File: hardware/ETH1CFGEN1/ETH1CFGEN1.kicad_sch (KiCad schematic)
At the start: 0 parts

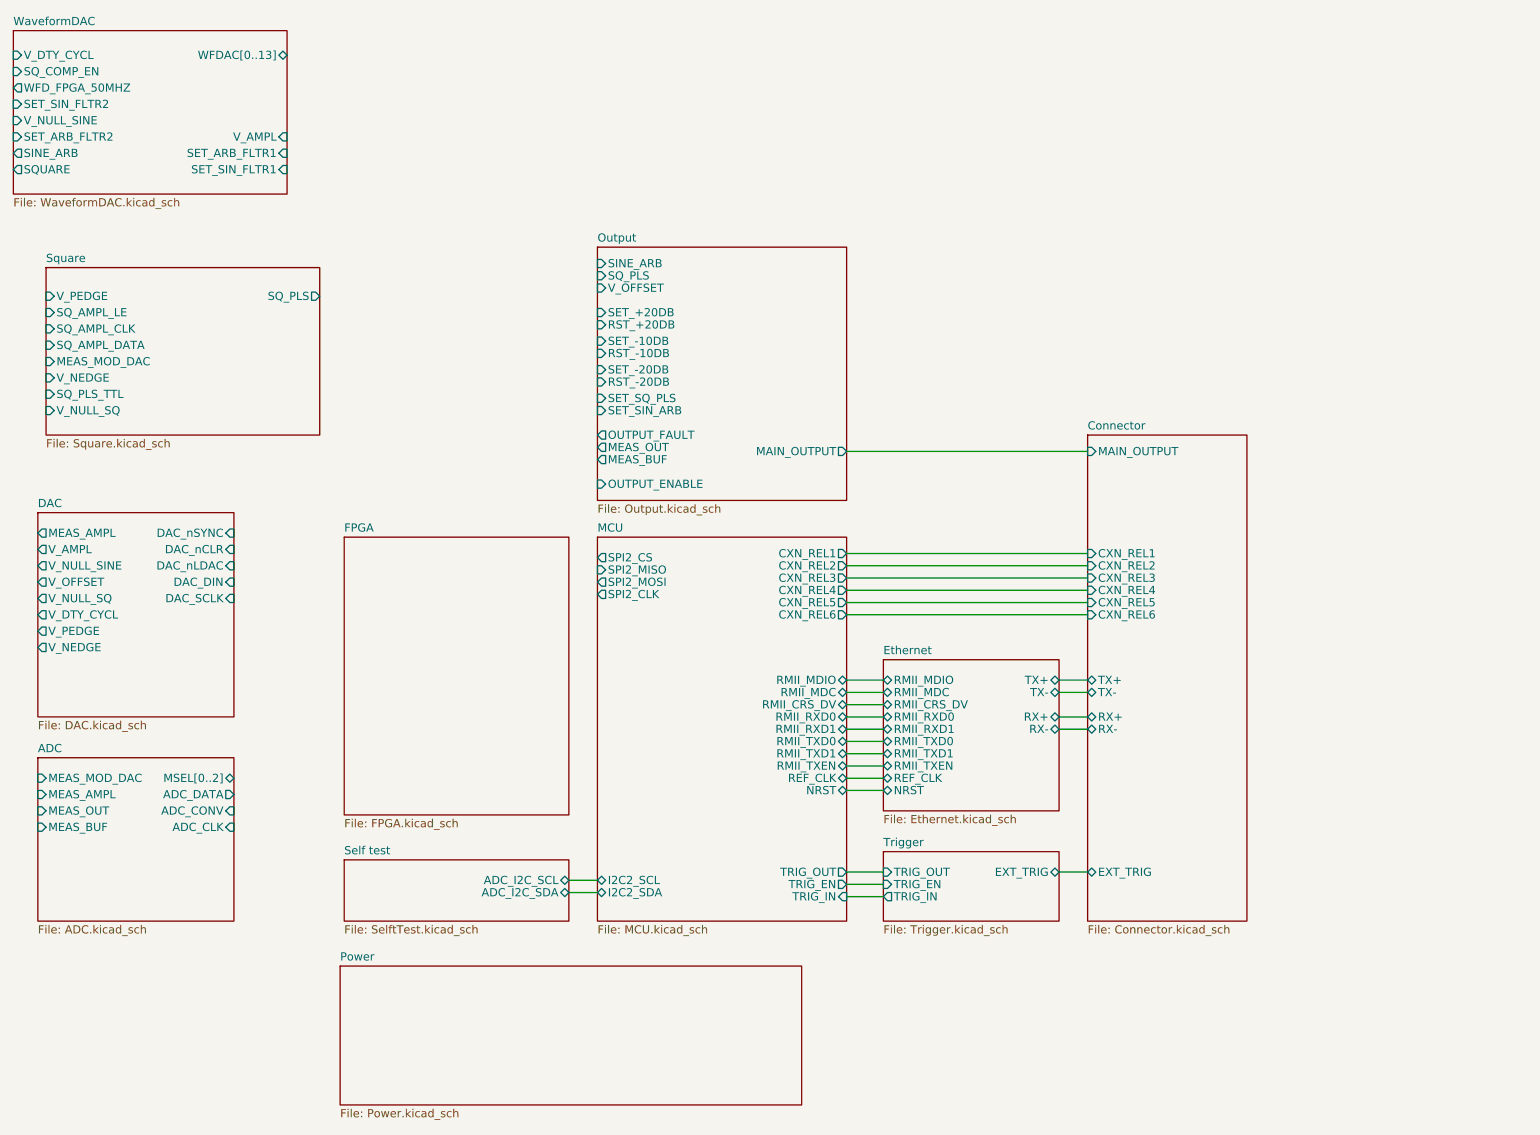
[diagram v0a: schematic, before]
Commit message: PCB design
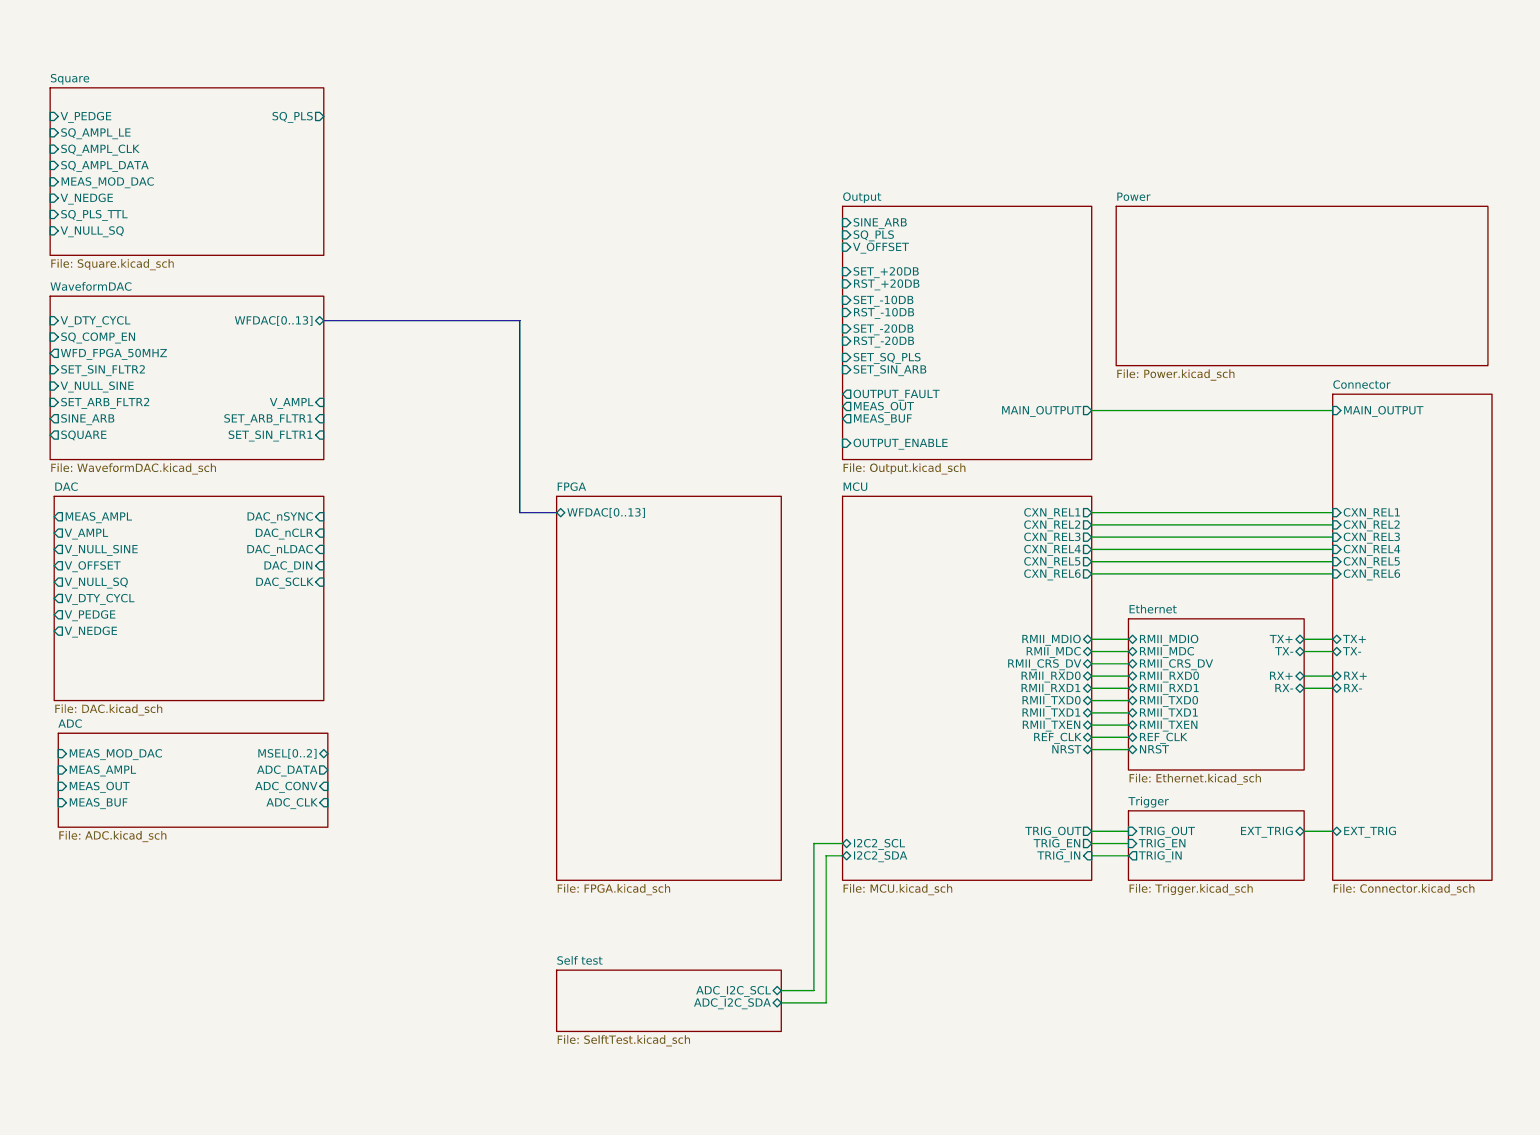
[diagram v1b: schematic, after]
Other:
- sheet FPGA ports: added WFDAC[0..13]; removed none
- sheet MCU ports: added none; removed SPI2_CLK, SPI2_CS, SPI2_MISO, SPI2_MOSI
